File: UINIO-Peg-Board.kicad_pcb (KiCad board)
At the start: 2 copper layers, 100 x 100 mm, 0 parts

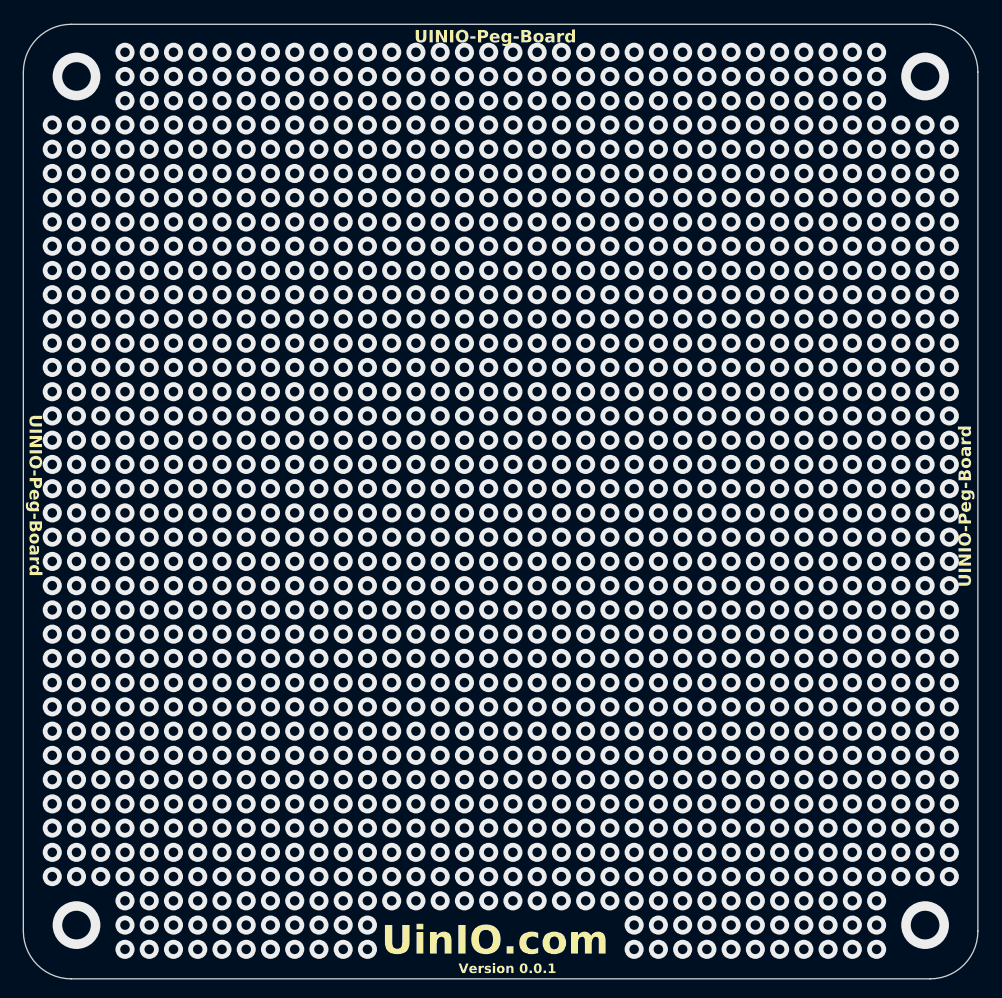
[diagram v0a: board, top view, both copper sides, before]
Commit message: Release UINIO-Peg-Board version 1.0.0.
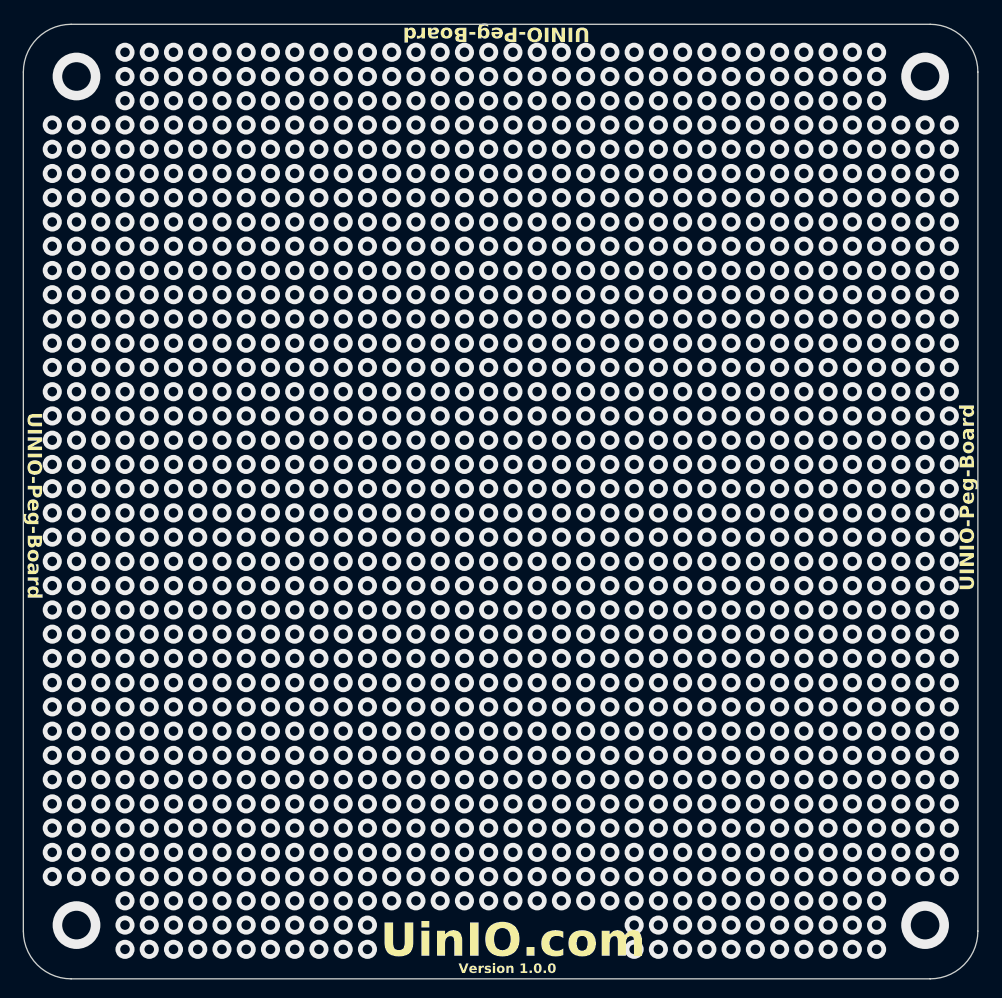
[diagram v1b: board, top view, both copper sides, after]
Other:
- board text added: "Version 1.0.0"
- board text removed: "Version 0.0.1"
